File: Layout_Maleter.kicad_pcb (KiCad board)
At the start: 4 copper layers, 112.4 x 104 mm, 74 parts, among them J1 Conn_01x02, J2 DB9_Male, J3 Conn_01x02, J4 Conn_01x02, J5 Conn_01x06_Fem, J6 Conn_Male, J7 Conn_01x02, K1 ADW11, K2 1393280-5, K3 1393280-5, Q1 BC817, Q2 BC817, Q3 BC817, U1 TCA39306DTMR, U2 MCP2551-I-P, U3 LM1117-5.0, U4 LM1117-3.3, U5 FDC2212QDNTTQ1, U6 PIC18F258-I/SP, U7 AD8616ARZ, Y1 Crystal

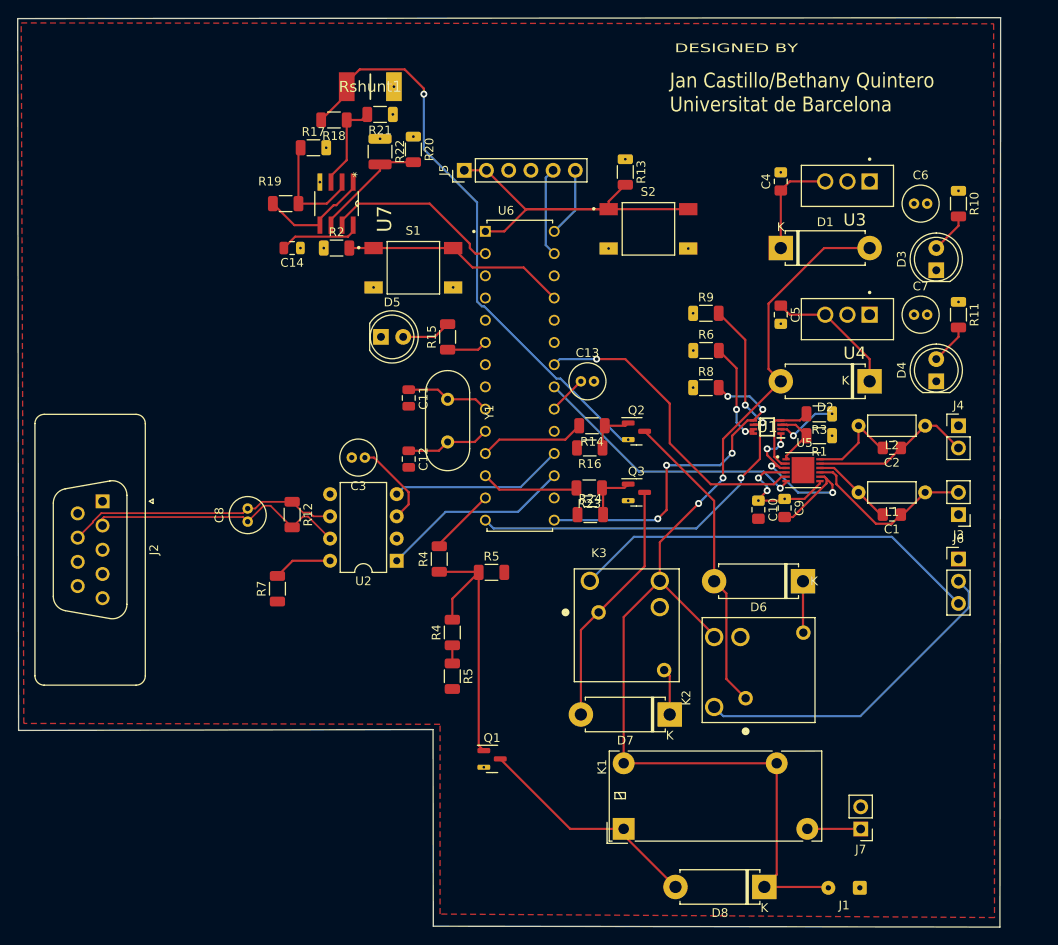
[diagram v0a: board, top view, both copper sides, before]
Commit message: Add files via upload
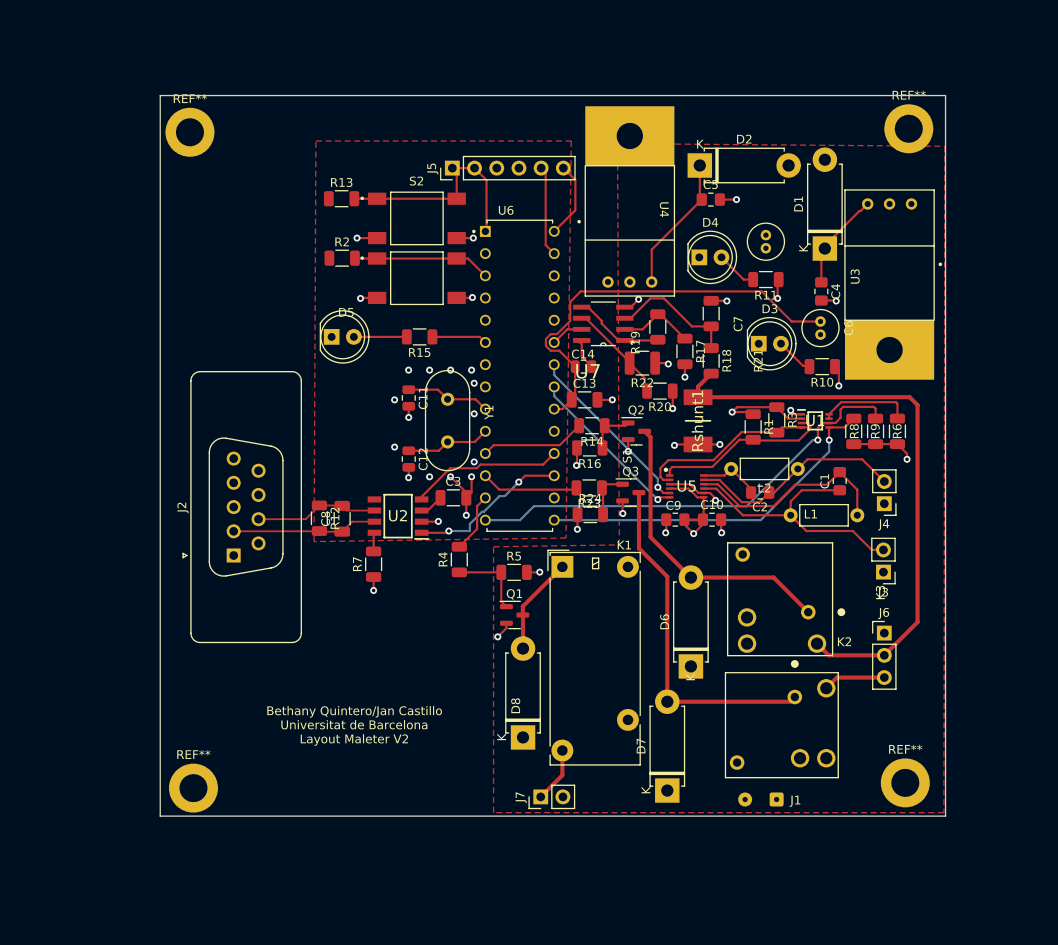
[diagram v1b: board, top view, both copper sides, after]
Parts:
- removed the R4 at (125.0, 110.0)
- removed the R5 at (125.0, 115.0)
- added REF**: MountingHole_3.2mm_M3_DIN965_Pad, MountingHole:MountingHole_3.2mm_M3_DIN965_Pad, F.Cu at (95.0, 52.8)
- added REF**: MountingHole_3.2mm_M3_DIN965_Pad, MountingHole:MountingHole_3.2mm_M3_DIN965_Pad, F.Cu at (95.4, 127.8)
- added REF**: MountingHole_3.2mm_M3_DIN965_Pad, MountingHole:MountingHole_3.2mm_M3_DIN965_Pad, F.Cu at (176.8, 127.2)
- added REF**: MountingHole_3.2mm_M3_DIN965_Pad, MountingHole:MountingHole_3.2mm_M3_DIN965_Pad, F.Cu at (177.2, 52.4)
- C13, C3, C8: footprint Capacitor_THT:C_Radial_D4.0mm_H5.0mm_P1.50mm -> Capacitor_SMD:C_1206_3216Metric
- U2: footprint Package_DIP:DIP-8_W7.62mm -> Llibreria_projecte:TRANSCEIVER_SMD
- U3, U4: footprint BQ_Library:TO254P1054X470X1955-3 -> BQ_Library:TO-220
- U5: footprint Llibreria_Projecte_Maleter:SON50P400X400X100-13N -> Llibreria_projecte:SON50P400X400X100-13N
- moved Rshunt1 53.5 mm to (153.1, 85.8), turned to -90 degrees
- moved R18 51.2 mm to (154.6, 78.9), turned to -90 degrees
- moved R17 48.5 mm to (151.6, 77.9), turned to -90 degrees
- moved R19 44.8 mm to (148.5, 75.1), turned to -90 degrees
- moved R21 44.2 mm to (154.6, 73.5), turned to -90 degrees
- moved R20 39.5 mm to (148.7, 82.4), turned to 180 degrees
- moved R22 38.5 mm to (146.7, 79.2), turned to 180 degrees
- moved J7 36.8 mm to (135.1, 128.8), turned to 90 degrees
- moved C14 36.0 mm to (140.0, 79.6), turned to 0 degrees
- moved U7 33.5 mm to (142.3, 74.7), turned to 180 degrees
- moved R13 32.6 mm to (112.3, 60.4), turned to 0 degrees
- moved D8 32.5 mm to (133.1, 122.0), turned to 90 degrees
- moved D2 31.4 mm to (153.3, 56.6), turned to 0 degrees
- moved K1 30.8 mm to (137.6, 102.5), turned to 0 degrees
- moved D4 30.6 mm to (153.2, 67.1), turned to 0 degrees
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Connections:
- D6 pad 1: Net-(D6-Pad1) -> VBAT
- D7 pad 1: Net-(D7-Pad1) -> VBAT
- K2 pad 2: Net-(D6-Pad1) -> VBAT
- K3 pad 2: Net-(D7-Pad1) -> VBAT
- Q2 pad 2: /Relé_Out -> GND
- R18 pad 2: /Relé_Out -> M1
- Rshunt1 pad 1: /Relé_Out -> M1
- U6 pad 2: INTERRP -> unconnected-(U6-Pad2)
- U6 pad 23: unconnected-(U6-Pad23) -> INTERRP
- U6 pad 25: /Heater -> unconnected-(U6-Pad25)
- U6 pad 3: unconnected-(U6-Pad3) -> /Heater
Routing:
- net VBAT: track 124.0 -> 0.00 mm, vias 2 -> 0
- net /Relé_Out: track 66.6 -> 0.00 mm, vias 1 -> 0
- net +VCC1: track 14.4 -> 60.3 mm, vias 0 -> 2
- net M2: track 47.4 -> 7.14 mm
- net GND: track 25.8 -> 59.8 mm, vias 4 -> 40
- net M1: track 38.2 -> 67.5 mm
- net Net-(Q1-Pad1): track 31.8 -> 9.06 mm
- net /RESET: track 46.7 -> 26.3 mm
- net /CAN-: track 31.3 -> 14.1 mm
- net INTERRP: track 20.4 -> 3.77 mm
- net Net-(D8-Pad2): track 26.5 -> 11.2 mm
- net /INTB: track 35.7 -> 20.6 mm
- net Net-(C1-Pad2): track 9.40 -> 24.0 mm
- net /CAN+: track 30.5 -> 17.0 mm
- net Net-(D7-Pad2): track 28.4 -> 41.0 mm
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- added copper zone on F.Cu, net +VCC1
- added copper zone on In1.Cu, net +VCC2
- added copper zone on In1.Cu, net GND
- added copper zone on In2.Cu, net GND
- added copper zone on F.Cu, net VBAT
- removed copper zone on In2.Cu, net +VCC2
- removed copper zone on F.Cu, net GND
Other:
- board size 112.4 x 104 mm -> 89.8 x 82.4 mm
- board text added: "Bethany Quintero/Jan Castillo Universitat de Barcelona Layout Maleter V2"
- board text removed: "DESIGNED BY"
- board text removed: "Jan Castillo/Bethany Quintero Universitat de Barcelona"

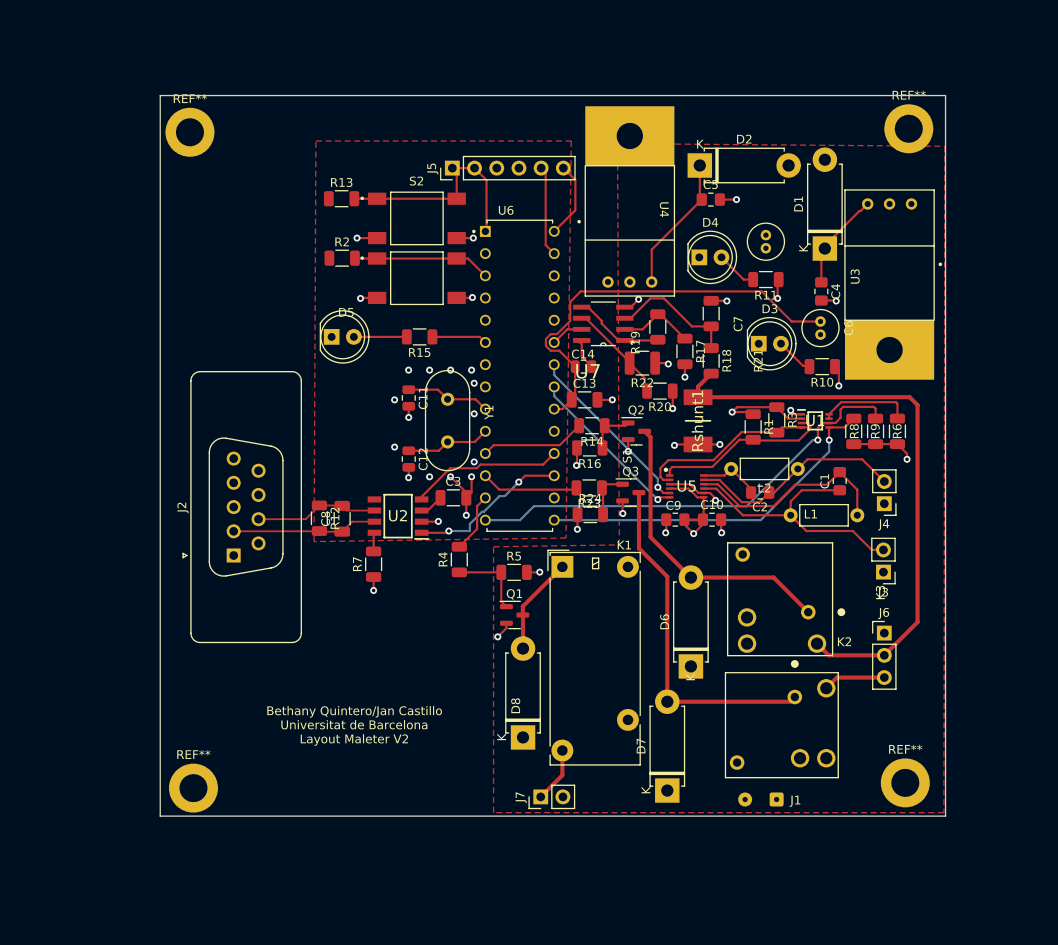
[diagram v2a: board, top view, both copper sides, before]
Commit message: Add files via upload
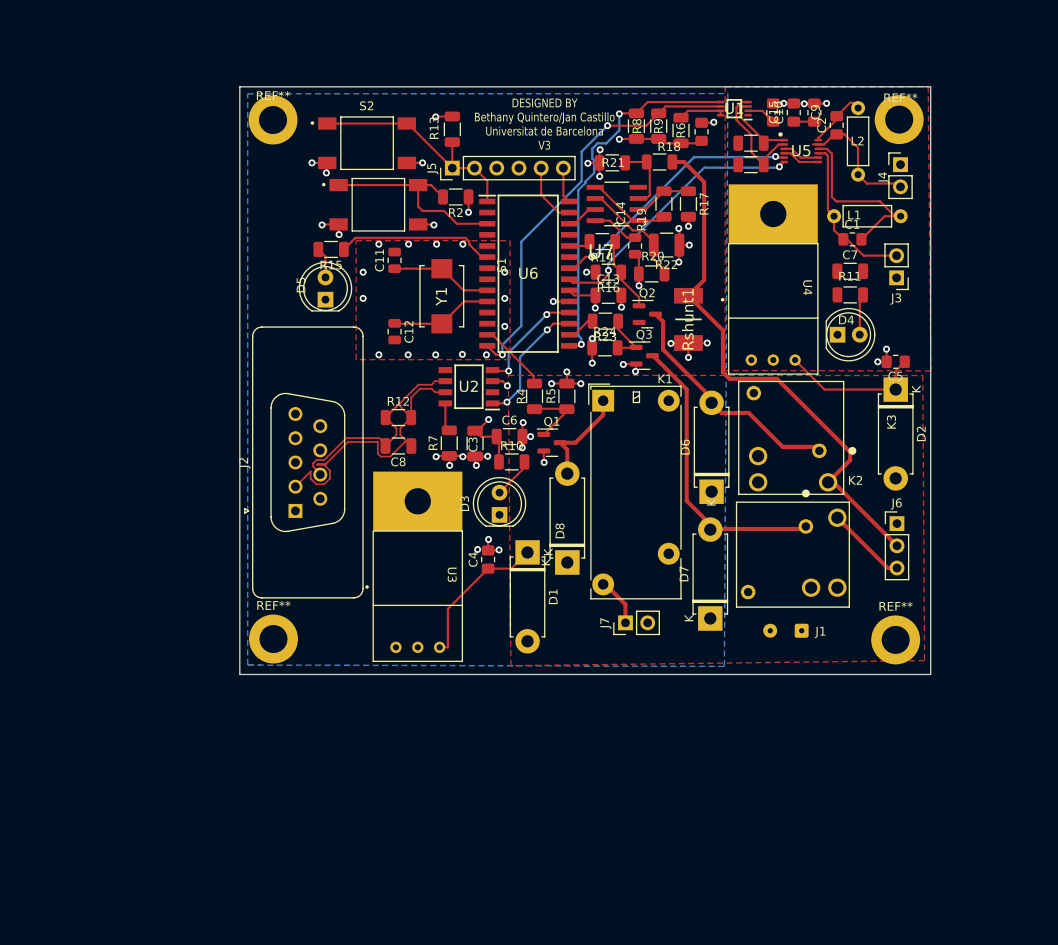
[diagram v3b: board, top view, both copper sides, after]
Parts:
- removed the REF** at (95.0, 52.8)
- removed the REF** at (95.4, 127.8)
- removed the REF** at (176.8, 127.2)
- removed the REF** at (177.2, 52.4)
- added C15: 0.1 uF, Capacitor_SMD:C_0805_2012Metric_Pad1.18x1.45mm_HandSolder, F.Cu at (161.7, 50.5)
- added C16: 0.1 uF, Capacitor_SMD:C_0805_2012Metric_Pad1.18x1.45mm_HandSolder, F.Cu at (153.5, 52.8)
- added REF**: MountingHole_3.2mm_M3_DIN965_Pad, MountingHole:MountingHole_3.2mm_M3_DIN965_Pad, F.Cu at (104.5, 51.4)
- added REF**: MountingHole_3.2mm_M3_DIN965_Pad, MountingHole:MountingHole_3.2mm_M3_DIN965_Pad, F.Cu at (104.5, 110.8)
- added REF**: MountingHole_3.2mm_M3_DIN965_Pad, MountingHole:MountingHole_3.2mm_M3_DIN965_Pad, F.Cu at (175.7, 110.8)
- added REF**: MountingHole_3.2mm_M3_DIN965_Pad, MountingHole:MountingHole_3.2mm_M3_DIN965_Pad, F.Cu at (176.1, 51.4)
- C6, C7: footprint Capacitor_THT:C_Radial_D4.0mm_H5.0mm_P1.50mm -> Capacitor_SMD:C_1206_3216Metric
- R22: value 80k -> 120k
- U6: footprint Llibreria_Projecte_Maleter:DIP787W45P254L3556H508Q28 -> Llibreria_projecte:MICROSMD
- Y1: footprint Crystal:Crystal_HC49-4H_Vertical -> Llibreria_projecte:CRISTALL
- moved U3 63.8 mm to (121.0, 103.4), turned to -90 degrees
- moved C9 49.2 mm to (166.4, 50.5), turned to 90 degrees
- moved C4 48.9 mm to (129.1, 101.7), turned to 90 degrees
- moved D1 48.6 mm to (133.6, 100.8), turned to -90 degrees
- moved C10 47.5 mm to (164.1, 50.5), turned to 90 degrees
- moved C2 42.9 mm to (168.9, 52.0), turned to 90 degrees
- moved R8 42.8 mm to (146.1, 52.1)
- moved R9 42.8 mm to (148.6, 52.1)
- moved R6 42.4 mm to (151.2, 52.6)
- moved U5 40.5 mm to (164.9, 55.0)
- moved J4 38.8 mm to (176.2, 56.5), turned to 0 degrees
- moved C6 37.9 mm to (131.6, 87.6), turned to 0 degrees
- moved R10 37.1 mm to (131.8, 90.5), turned to 0 degrees
- moved U1 36.9 mm to (157.2, 50.1), turned to 180 degrees
- moved D3 35.5 mm to (130.4, 96.5), turned to 90 degrees
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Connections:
- R20 pad 1: +VCC2 -> +VCC1
- U3 pad 4: +VCC1 -> (no net)
- U4 pad 4: +VCC2 -> (no net)
- U6 pad 11: /Relé1 -> unconnected-(U6-Pad11)
- U6 pad 12: /Relé2 -> unconnected-(U6-Pad12)
- U6 pad 16: unconnected-(U6-Pad16) -> /Relé2
- U6 pad 23: INTERRP -> unconnected-(U6-Pad23)
- U6 pad 24: unconnected-(U6-Pad24) -> /Relé1
- U6 pad 26: unconnected-(U6-Pad26) -> INTERRP
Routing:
- net +VCC1: track 60.3 -> 31.7 mm, vias 2 -> 7
- net +VCC2: track 29.3 -> 10.6 mm, vias 4 -> 0
- net /CAN+: track 17.0 -> 35.6 mm
- net /CAN-: track 14.1 -> 28.3 mm
- net Net-(C1-Pad1): track 31.2 -> 18.4 mm
- net /SD: track 19.3 -> 31.2 mm, vias 1 -> 2
- net Net-(R15-Pad1): track 6.32 -> 18.0 mm
- net /SCL1: track 20.2 -> 8.83 mm
- net GND: track 59.8 -> 70.4 mm, vias 40 -> 58
- net Net-(C2-Pad1): track 24.8 -> 14.8 mm
- net /Relé1: track 12.0 -> 2.54 mm
- net /INTB: track 20.6 -> 29.9 mm, vias 1 -> 2
- net /Heater: track 15.8 -> 23.7 mm
- net /SDA1: track 20.9 -> 13.0 mm
- net /Relé2: track 11.2 -> 3.33 mm
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- added copper zone on B.Cu, net +VCC1
- added copper zone on F.Cu, net +VCC2
- added copper zone on F.Cu, net GND
- removed copper zone on F.Cu, net +VCC1
- removed copper zone on In1.Cu, net +VCC1
- removed copper zone on In1.Cu, net +VCC2
- removed copper zone on In1.Cu, net GND
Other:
- board size 89.8 x 82.4 mm -> 79 x 67.2 mm
- board text added: "DESIGNED BY Bethany Quintero/Jan Castillo Universitat de Barcelona V3"
- board text removed: "Bethany Quintero/Jan Castillo Universitat de Barcelona Layout Maleter V2"
